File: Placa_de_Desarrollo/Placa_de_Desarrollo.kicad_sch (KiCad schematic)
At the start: 30 parts, among them J1 USB_A, J2 LEFT, J3 RIGHT, SW1 RESET, U1 LM317_TO-220, U2 RP2350

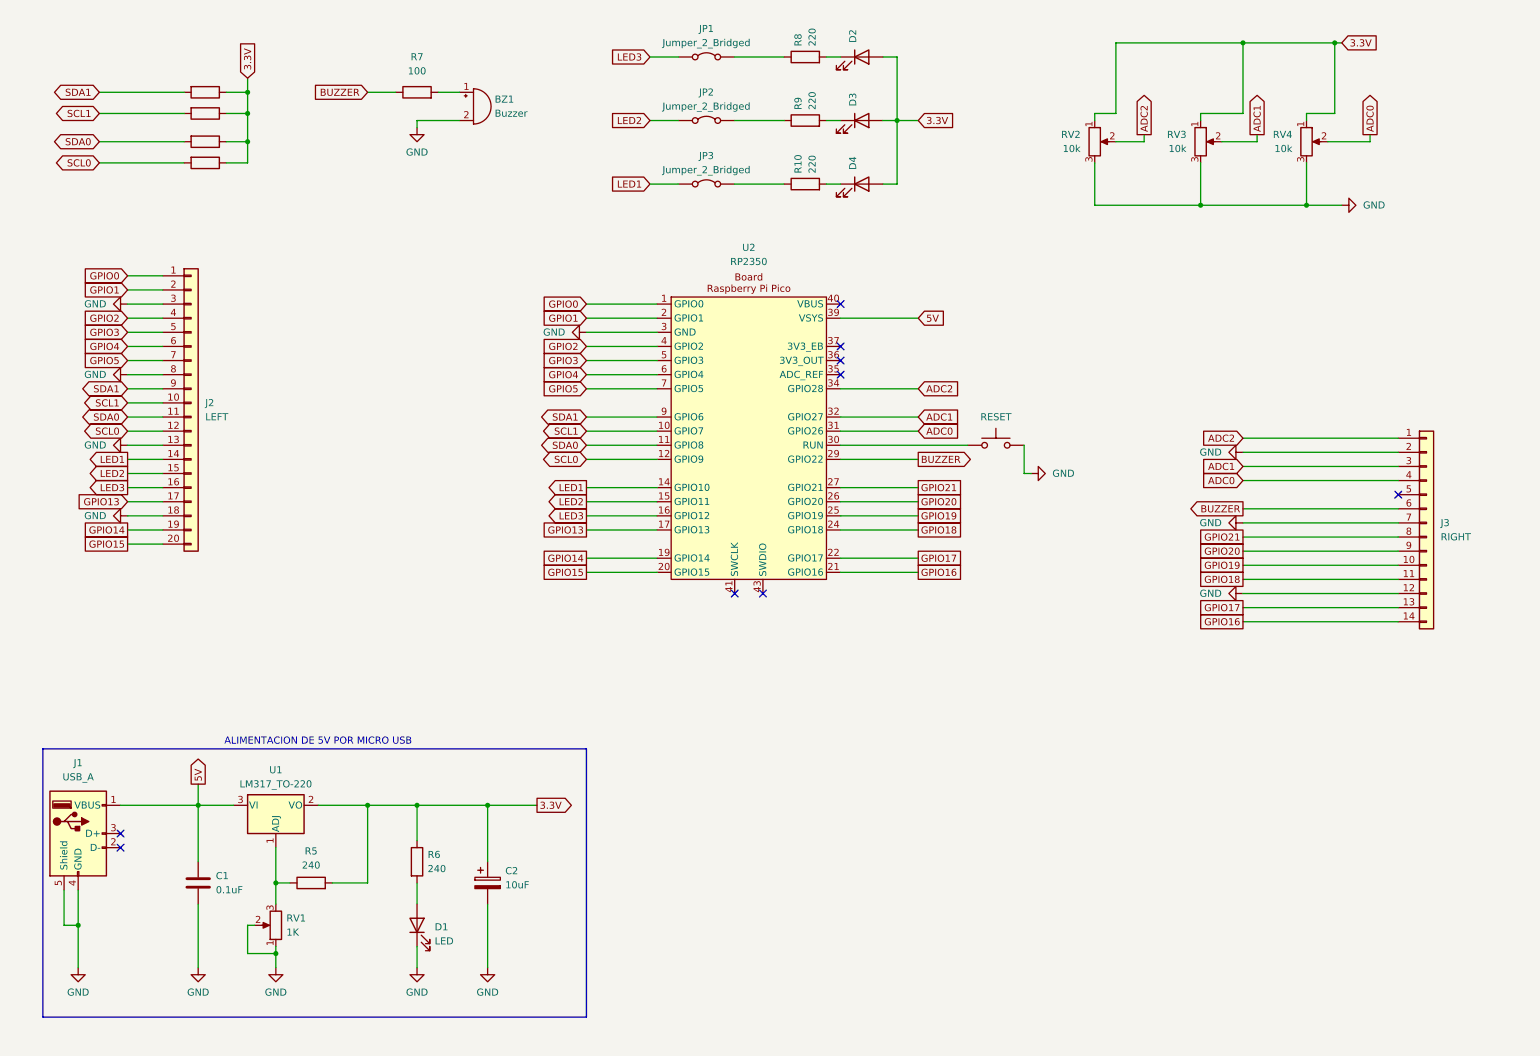
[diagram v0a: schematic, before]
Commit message: Version 2.0 de la Placa de DEsarrollo
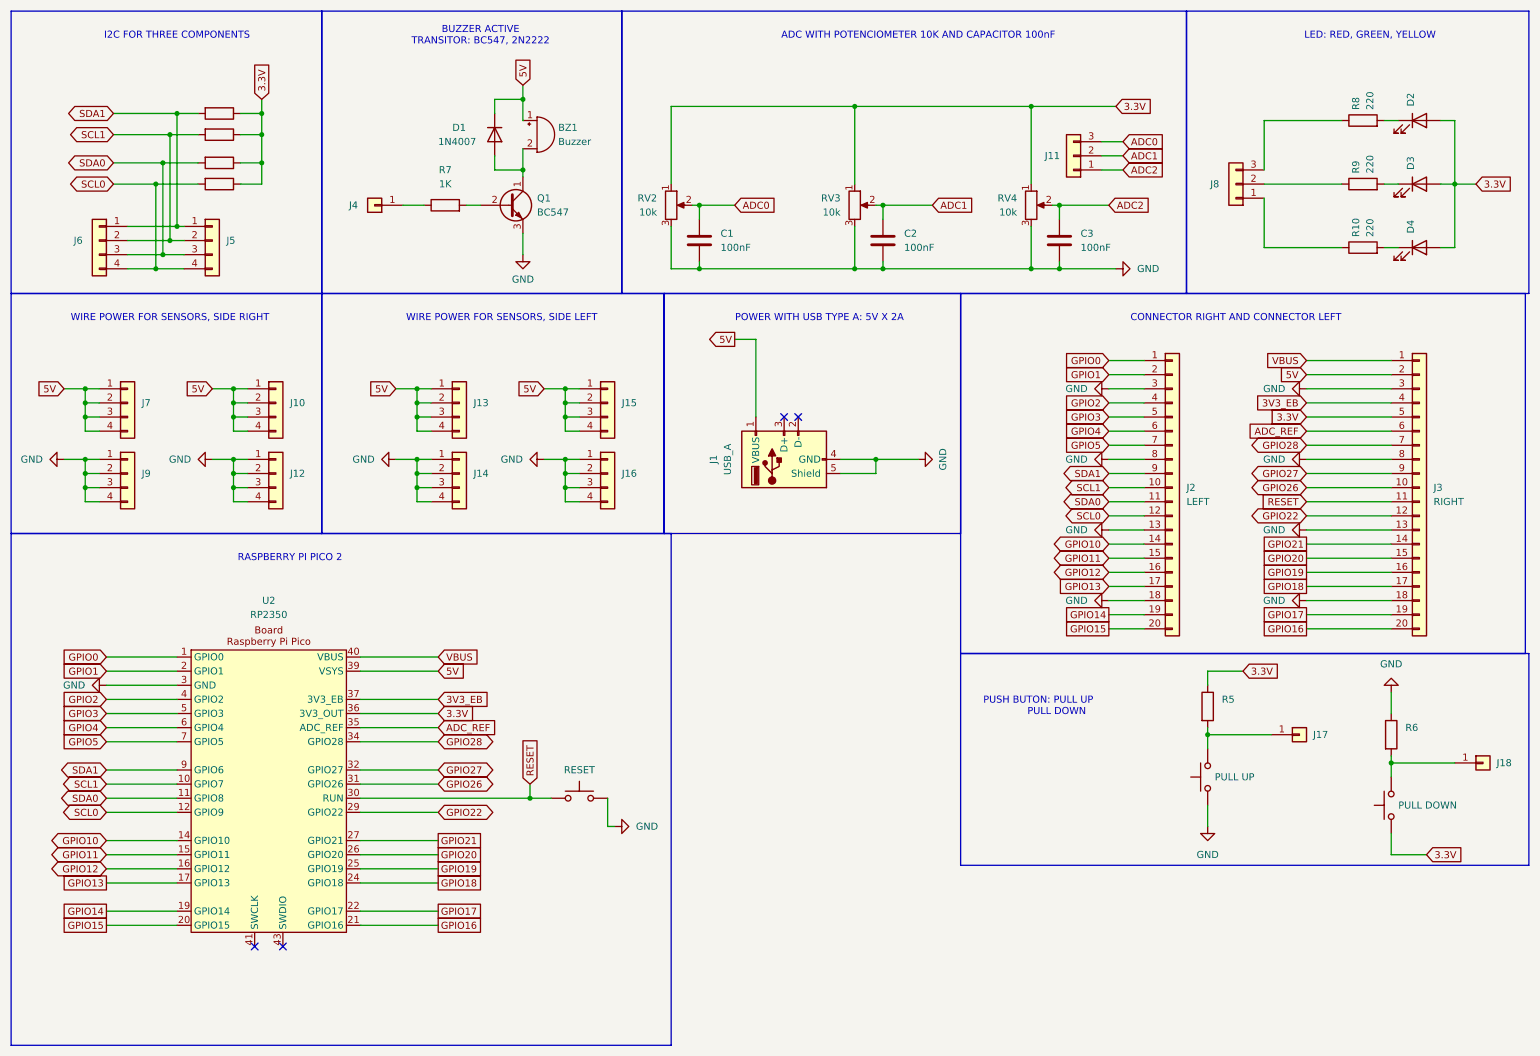
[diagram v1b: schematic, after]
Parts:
- removed C2: 10uF, Capacitor_THT:CP_Radial_D5.0mm_P2.00mm, symbol Device:C_Polarized
- removed D1: LED, LED_THT:LED_D5.0mm, symbol Device:LED
- removed JP1, JP2, JP3: Jumper_2_Bridged, Connector_PinHeader_2.54mm:PinHeader_1x02_P2.54mm_Vertical, symbol Jumper:Jumper_2_Bridged
- removed RV1: 1K, Potentiometer_THT:Potentiometer_Bourns_3296W_Vertical, symbol Device:R_Potentiometer
- removed U1: LM317_TO-220, Package_TO_SOT_THT:TO-220-3_Vertical, symbol Regulator_Linear:LM317_TO-220
- added C2, C3: 100nF, Capacitor_THT:C_Disc_D8.0mm_W2.5mm_P5.00mm, symbol Device:C
- added D1: 1N4007, Diode_THT:D_DO-41_SOD81_P10.16mm_Horizontal, symbol Diode:1N4007
- added J10, J12, J13, J14, J15, J16, J5, J6, J7, J9: Conn_01x04, Connector_PinHeader_2.54mm:PinHeader_1x04_P2.54mm_Vertical, symbol Connector_Generic:Conn_01x04
- added J11, J8: Conn_01x03, Connector_PinHeader_2.54mm:PinHeader_1x03_P2.54mm_Vertical, symbol Connector_Generic:Conn_01x03
- added J17, J18, J4: Conn_01x01, Connector_PinHeader_2.54mm:PinHeader_1x01_P2.54mm_Vertical, symbol Connector_Generic:Conn_01x01
- added Q1: BC547, Package_TO_SOT_THT:TO-92_Inline, symbol Transistor_BJT:BC547
- added SW2: PULL DOWN, Button_Switch_THT:SW_PUSH_6mm, symbol Switch:SW_Push
- added SW3: PULL UP, Button_Switch_THT:SW_PUSH_6mm, symbol Switch:SW_Push
- C1: value 0.1uF -> 100nF; footprint Capacitor_THT:C_Disc_D5.0mm_W2.5mm_P5.00mm -> Capacitor_THT:C_Disc_D8.0mm_W2.5mm_P5.00mm
- J3: footprint Connector_PinHeader_2.54mm:PinHeader_1x14_P2.54mm_Vertical -> Connector_PinHeader_2.54mm:PinHeader_1x20_P2.54mm_Vertical; symbol Connector_Generic:Conn_01x14 -> Connector_Generic:Conn_01x20
- R5, R6: value 240 -> 10K
- R7: value 100 -> 1K
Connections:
- net 3.3V: now also J3.5 (Pin_5), R5.1, U2.36 (3V3_OUT), SW2.1; no longer R5.2, R6.1
- net 5V: now also BZ1.1 (+), J3.2 (Pin_2), D1.1 (K), J10.1 (Pin_1), J10.2 (Pin_2), J10.3 (Pin_3), J10.4 (Pin_4), J13.1 (Pin_1), J13.2 (Pin_2), J13.3 (Pin_3), J13.4 (Pin_4), J15.1 (Pin_1), J15.2 (Pin_2), J15.3 (Pin_3), J15.4 (Pin_4), J7.1 (Pin_1), J7.2 (Pin_2), J7.3 (Pin_3), J7.4 (Pin_4); no longer C1.1
- net ADC0: now also C1.1, RV2.2, J11.3 (Pin_3); no longer J3.4 (Pin_4), RV4.2, U2.31 (GPIO26)
- net ADC1: now also C2.1, J11.2 (Pin_2); no longer J3.3 (Pin_3), U2.32 (GPIO27)
- net ADC2: now also RV4.2, C3.1, J11.1 (Pin_1); no longer J3.1 (Pin_1), RV2.2, U2.34 (GPIO28)
- net GND: now also J3.13 (Pin_13), J3.18 (Pin_18), J3.3 (Pin_3), J3.8 (Pin_8), R6.1, C2.2, C3.2, J12.1 (Pin_1), J12.2 (Pin_2), J12.3 (Pin_3), J12.4 (Pin_4), J14.1 (Pin_1), J14.2 (Pin_2), J14.3 (Pin_3), J14.4 (Pin_4), J16.1 (Pin_1), J16.2 (Pin_2), J16.3 (Pin_3), J16.4 (Pin_4), J9.1 (Pin_1), J9.2 (Pin_2), J9.3 (Pin_3), J9.4 (Pin_4), Q1.3 (E), SW3.1; no longer BZ1.2 (-), J3.12 (Pin_12), J3.2 (Pin_2), J3.7 (Pin_7)
- net GPIO16: now also J3.20 (Pin_20); no longer J3.14 (Pin_14)
- net GPIO17: now also J3.19 (Pin_19); no longer J3.13 (Pin_13)
- net GPIO18: now also J3.17 (Pin_17); no longer J3.11 (Pin_11)
- net GPIO19: now also J3.16 (Pin_16); no longer J3.10 (Pin_10)
- net GPIO20: now also J3.15 (Pin_15); no longer J3.9 (Pin_9)
- net GPIO21: now also J3.14 (Pin_14); no longer J3.8 (Pin_8)
- net SCL0: now also J5.4 (Pin_4), J6.4 (Pin_4)
- net SCL1: now also J5.2 (Pin_2), J6.2 (Pin_2)
- net SDA0: now also J5.3 (Pin_3), J6.3 (Pin_3)
- net SDA1: now also J5.1 (Pin_1), J6.1 (Pin_1)
- net at R8.1: now also J8.3 (Pin_3)
- net at R7.2: now also Q1.2 (B); no longer BZ1.1 (+)
- net at R9.1: now also J8.2 (Pin_2)
- net at R6.2: now also J18.1 (Pin_1), SW2.2
- net RESET: now reaches SW1.1, U2.30 (RUN)
- net RESET: now also J3.11 (Pin_11)
- net ADC_REF: now reaches U2.35 (ADC_REF)
- net ADC_REF: now also J3.6 (Pin_6)
- net 3V3_EB: now reaches U2.37 (3V3_EB)
- net 3V3_EB: now also J3.4 (Pin_4)
- net VBUS: now reaches U2.40 (VBUS)
- net VBUS: now also J3.1 (Pin_1)
- net at R10.1: now also J8.1 (Pin_1)
- removed net BUZZER: J3.6 (Pin_6), R7.1, U2.29 (GPIO22)
- net LED1 renamed GPIO10
- net LED2 renamed GPIO11
- net LED3 renamed GPIO12
- new net: J4.1 (Pin_1), R7.1
- new net: BZ1.2 (-), D1.2 (A), Q1.1 (C)
- new net: J17.1 (Pin_1), R5.2, SW3.2
- new net GPIO22: J3.12 (Pin_12), U2.29 (GPIO22)
- new net GPIO26: J3.10 (Pin_10), U2.31 (GPIO26)
- new net GPIO27: J3.9 (Pin_9), U2.32 (GPIO27)
- new net GPIO28: J3.7 (Pin_7), U2.34 (GPIO28)
- no-connect marks 9 -> 4
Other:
- note added: "ADC WITH POTENCIOMETER 10K AND CAPACITOR 100nF"
- note added: "BUZZER ACTIVE TRANSITOR: BC547, 2N2222"
- note added: "CONNECTOR RIGHT AND CONNECTOR LEFT"
- note added: "I2C FOR THREE COMPONENTS"
- note added: "LED: RED, GREEN, YELLOW"
- note added: "POWER WITH USB TYPE A: 5V X 2A"
- note added: "PUSH BUTON: PULL UP PULL DOWN"
- note added: "RASPBERRY PI PICO 2"
- note added: "WIRE POWER FOR SENSORS, SIDE LEFT"
- note added: "WIRE POWER FOR SENSORS, SIDE RIGHT"
- note removed: "ALIMENTACION DE 5V POR MICRO USB"
- moved on the sheet: BZ1, D2, D3, D4, J1, J2, R10, R7, R8, R9, RV2, RV3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
